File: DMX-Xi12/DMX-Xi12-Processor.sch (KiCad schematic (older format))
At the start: 15 parts, among them U1 LPC11U68JBD100E

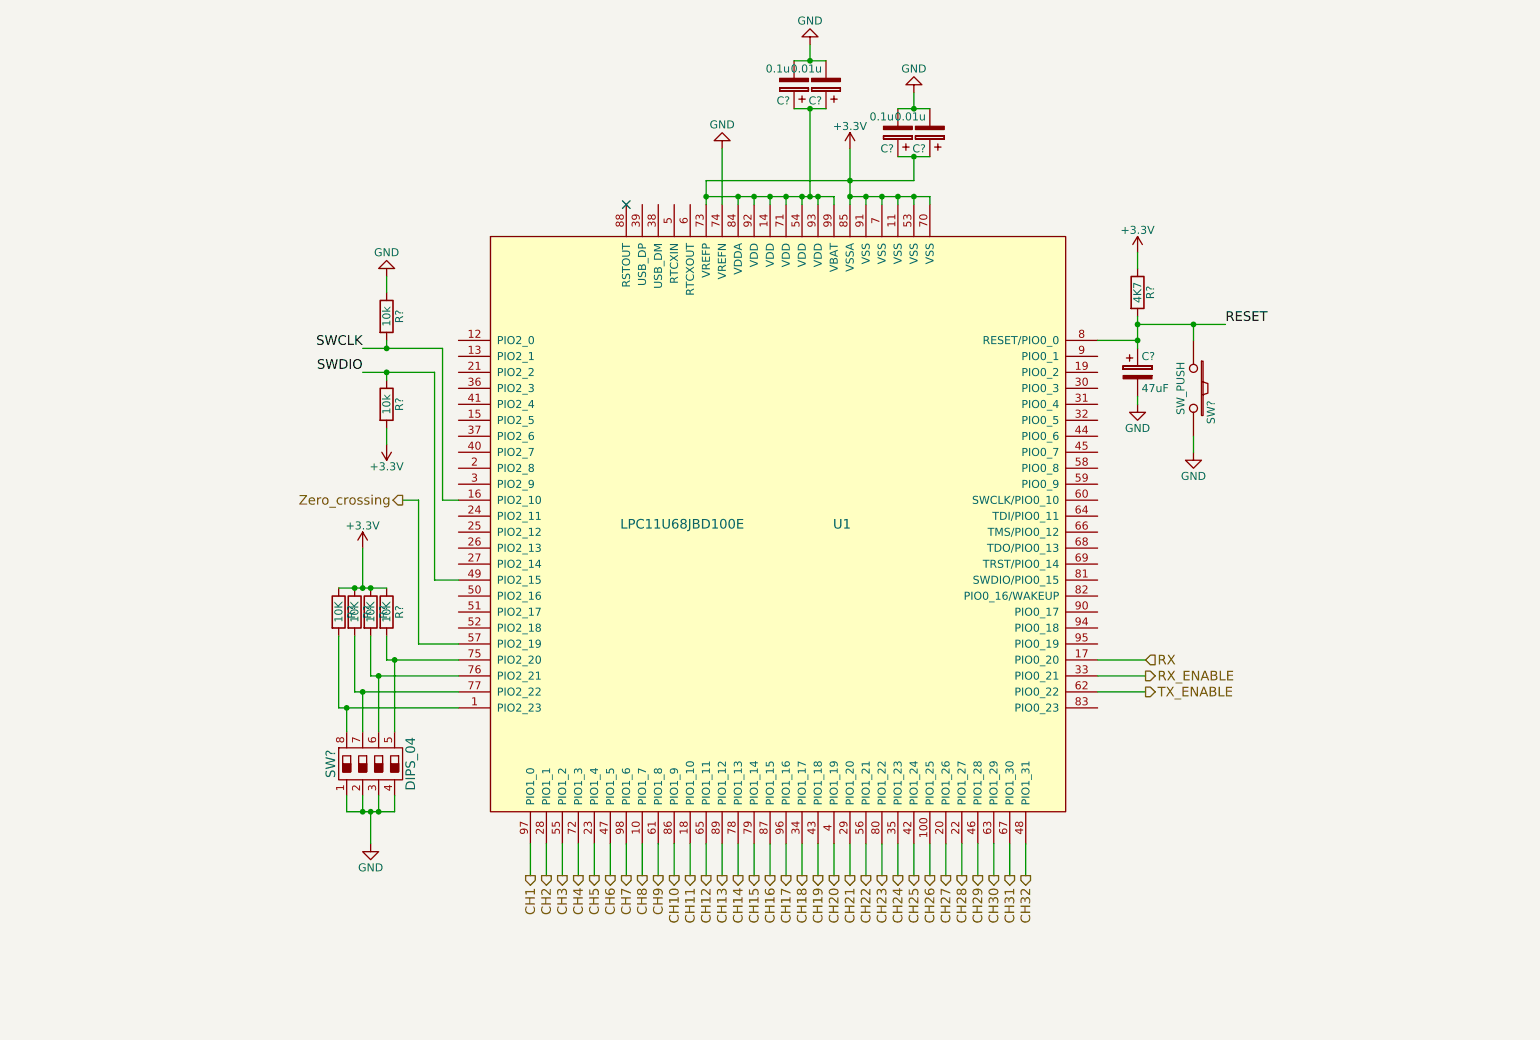
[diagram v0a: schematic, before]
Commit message: made dlaw changes etc
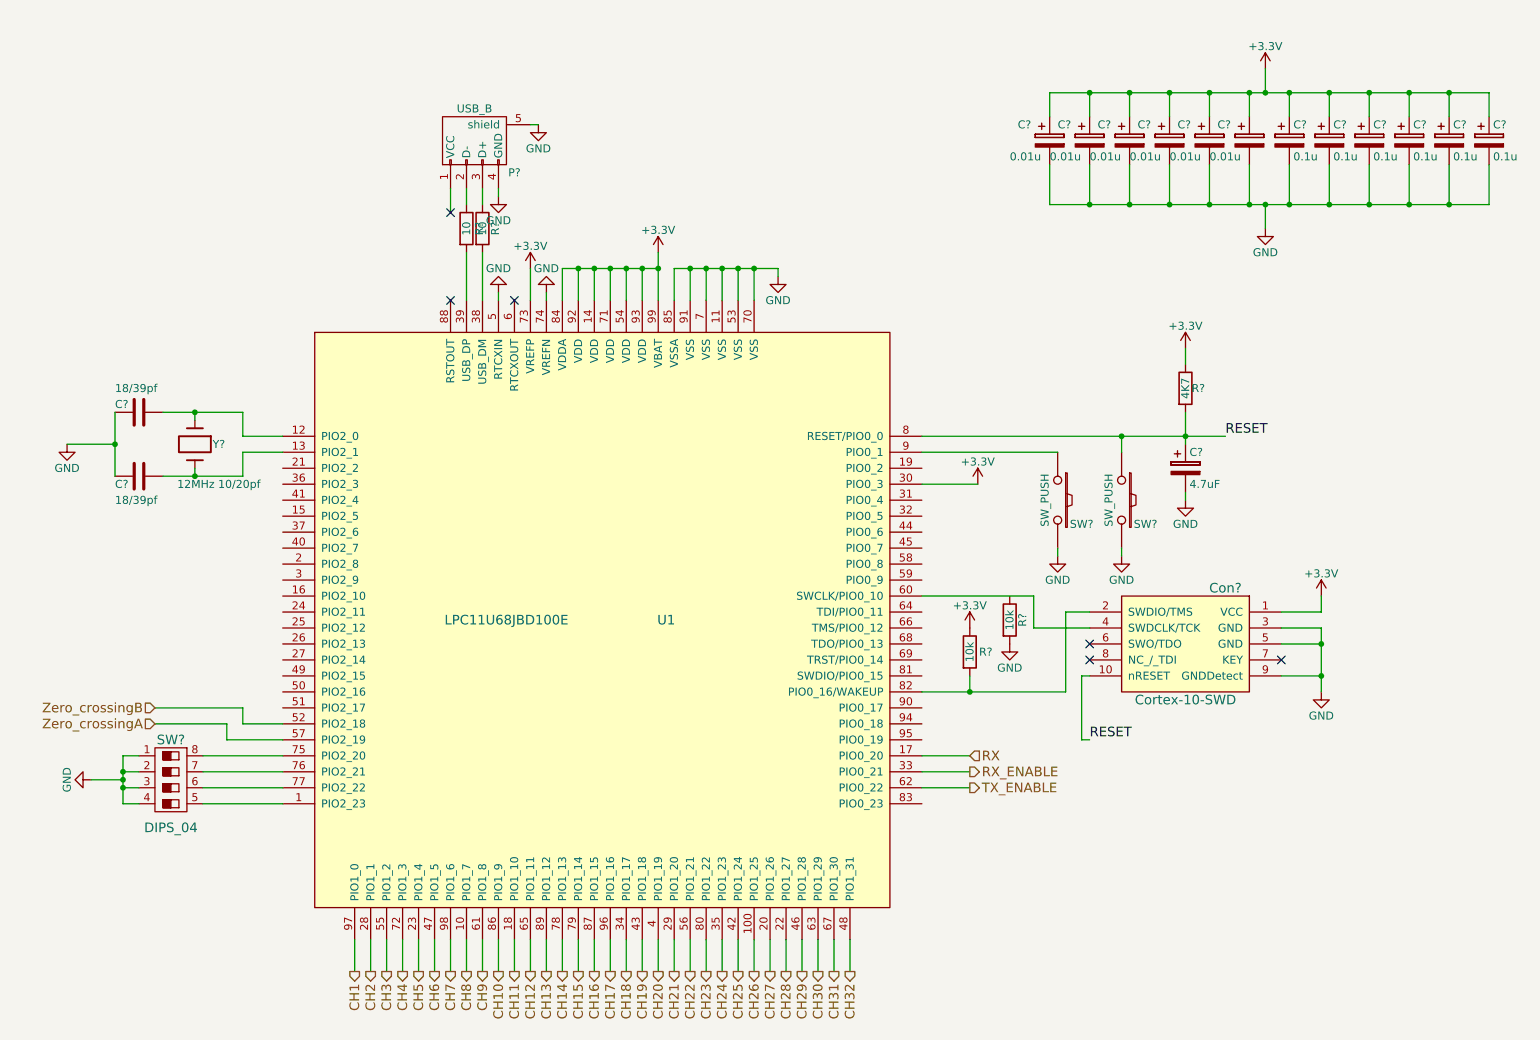
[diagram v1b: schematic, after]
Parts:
- removed C?: 0.1u, symbol CP
- removed C?: 0.01u, symbol CP
- removed R? (x4): 10K, symbol R
- removed R? (x2): 10k, symbol R
- added C? (x2): 18/39pf, symbol C
- added C? (x5): 0.1u, symbol CP
- added C? (x5): 0.01u, symbol CP
- added Con?: Cortex-10-SWD, symbol Cortex-10-SWD
- added P?: USB_B, symbol USB_B
- added R? (x2): 10, symbol R
- added R? (x2): 10k, symbol R
- added SW?: SW_PUSH, symbol SW_PUSH
- added Y?: 12MHz 10/20pf, symbol Crystal
- C?: value 47uF -> 4.7uF
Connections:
- net +3V3: now also U1.30 (PIO0_3), C?.1, C?.1, C?.1, C?.1, C?.1, C?.1, C?.1, C?.1, C?.1, C?.1, Con?.1 (VCC), R?.1; no longer U1.11 (VSS), U1.53 (VSS), U1.7 (VSS), U1.70 (VSS), U1.85 (VSSA), U1.91 (VSS)
- net GND: now also U1.11 (VSS), U1.5 (RTCXIN), U1.53 (VSS), U1.7 (VSS), U1.70 (VSS), U1.85 (VSSA), U1.91 (VSS), C?.2, C?.2, C?.2, C?.2, C?.2, C?.2, C?.2, C?.2, C?.2, C?.2, C?.2, C?.2, Con?.3 (GND), Con?.5 (GND), Con?.9 (GNDDetect), P?.4 (GND), P?.5 (shield), R?.2, SW?.2
- net RESET: now also Con?.10 (nRESET)
- net at U1.1 (PIO2_23): now also SW?.5; no longer SW?.8
- net at U1.12 (PIO2_0): now also C?.1, Y?.1
- net at U1.13 (PIO2_1): now also C?.1, Y?.2
- net at U1.38 (USB_DM): now also R?.2
- net at U1.39 (USB_DP): now also R?.2
- net Zero_crossingB: now reaches U1.52 (PIO2_18)
- net at U1.60 (SWCLK/PIO0_10): now also Con?.4 (SWDCLK/TCK)
- net at U1.75 (PIO2_20): now also SW?.8; no longer SW?.5
- net at U1.76 (PIO2_21): now also SW?.7; no longer SW?.6
- net at U1.77 (PIO2_22): now also SW?.6; no longer SW?.7
- net at U1.82 (PIO0_16/WAKEUP): now also Con?.2 (SWDIO/TMS), R?.2
- net at U1.9 (PIO0_1): now also SW?.1
- net SWCLK: no longer names the net of U1.16 (PIO2_10)
- net SWDIO: no longer names the net of U1.49 (PIO2_15)
- net Zero_crossing renamed Zero_crossingA
- new net: P?.2 (D-), R?.1
- new net: P?.3 (D+), R?.1
- no-connect marks 1 -> 6
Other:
- moved on the sheet: C?, R?, SW?, U1
